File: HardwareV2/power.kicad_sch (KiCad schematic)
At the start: 15 parts, among them CN1 S2B-PH-SM4-TB(LF)(SN), SW1 SW_SPDT, U2 BQ24040DSQR, U3 TPS63021DSJR

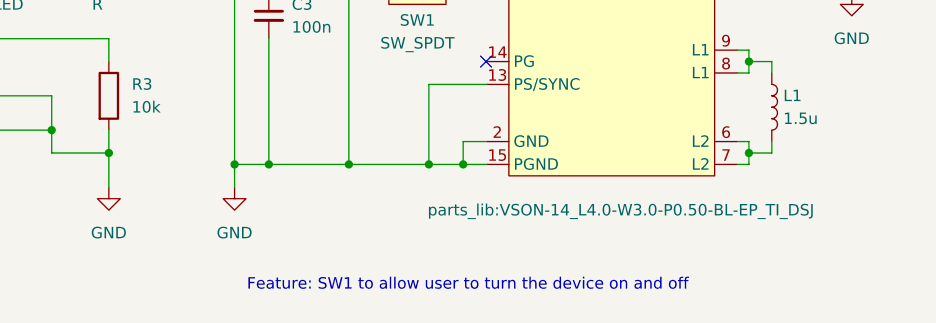
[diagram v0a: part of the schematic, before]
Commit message: commiting before flight :), added in crystal and started doing the labels for the RP2350b
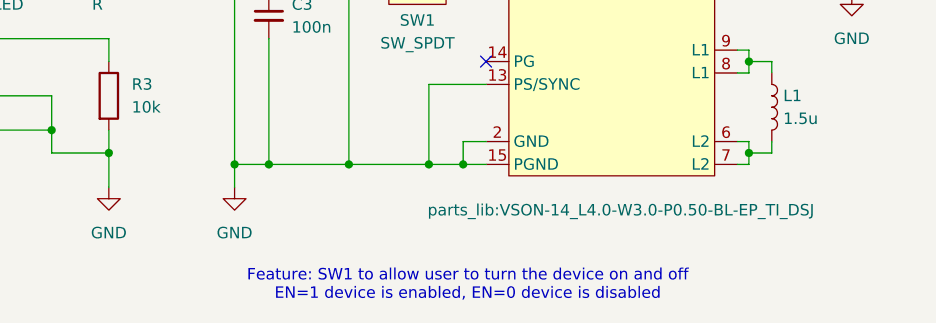
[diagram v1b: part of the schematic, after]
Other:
- note added: "Feature: SW1 to allow user to turn the device on and off EN=1 device is enabled, EN=0 device is disabled"
- note removed: "Feature: SW1 to allow user to turn the device on and off"
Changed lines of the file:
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@@
 		)
 	)
-	(text "Feature: SW1 to allow user to turn the device on and off"
+	(text "Feature: SW1 to allow user to turn the device on and off\nEN=1 device is enabled, EN=0 device is disabled"
 		(exclude_from_sim no)
 		(at 160.528 93.472 0)
